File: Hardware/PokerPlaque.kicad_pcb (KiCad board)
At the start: 2 copper layers, 43.1 x 40.2 mm, 10 parts, among them J1 A2541WR-5P, J2 A2541WR-4P, J3 A2541WR-2P, J4 A2541WR-8P, SW1 KH-6X6X6H-STM, U1 CH32V203C8T6

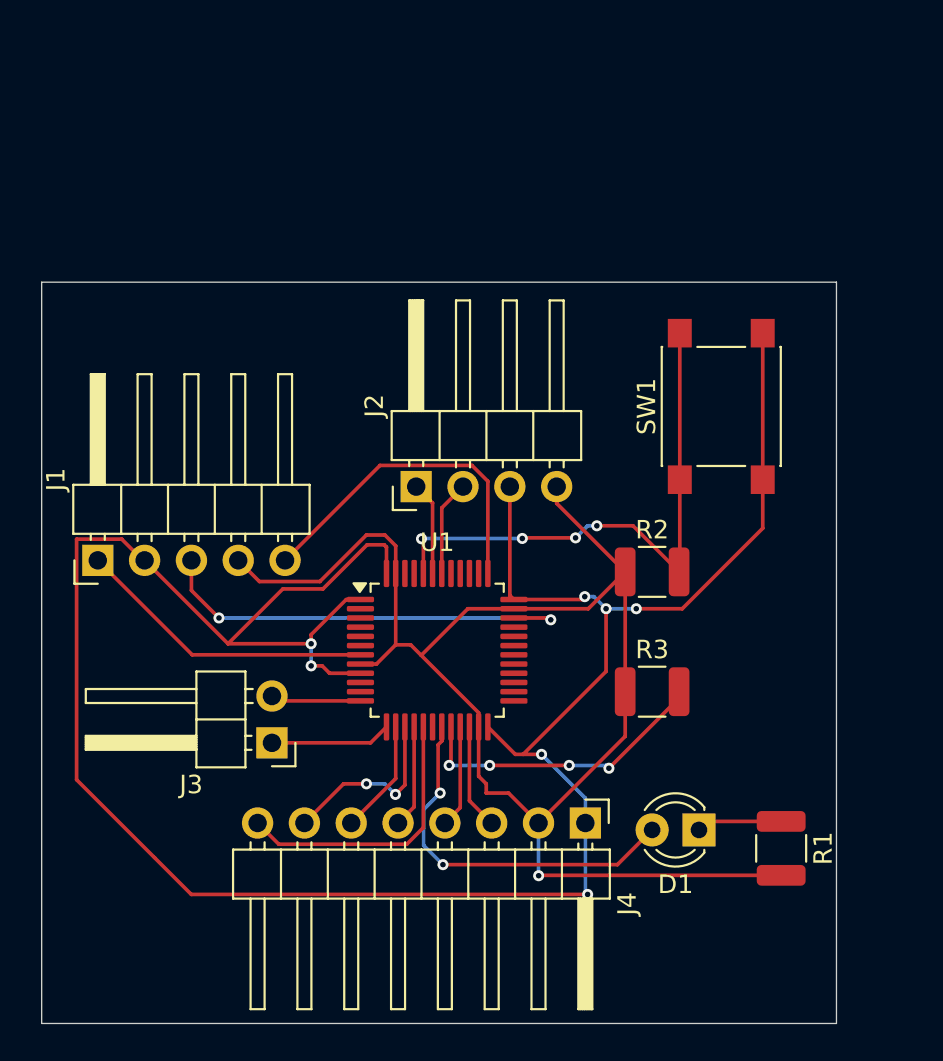
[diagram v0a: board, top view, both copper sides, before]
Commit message: feat: more things
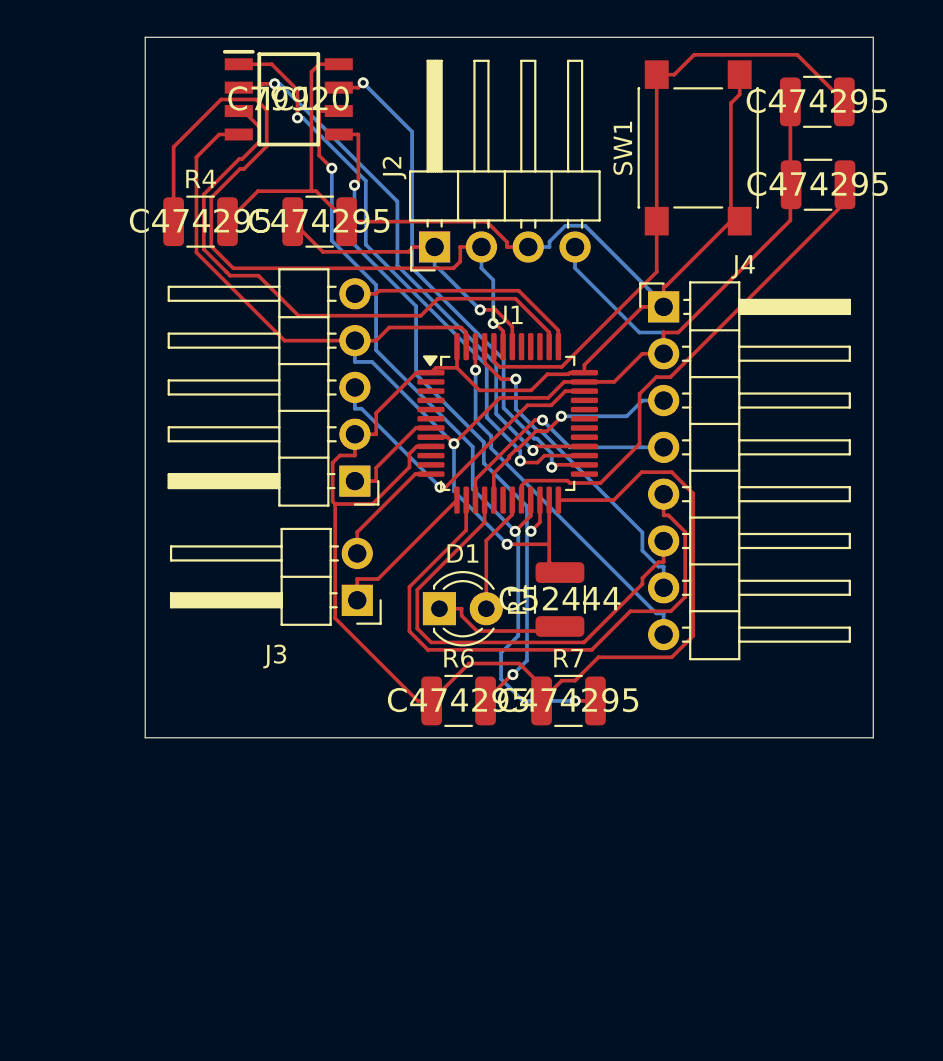
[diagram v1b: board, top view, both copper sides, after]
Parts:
- added IC1: M24C32-RMN6TP, M24C32-RMN6TP:SOIC127P600X175-8N, F.Cu at (35.3, 18.9)
- added R4: 1210W2J0103T5E, Resistor_SMD:R_1210_3225Metric, F.Cu at (30.5, 25.5)
- added R5: 1210W2J0103T5E, Resistor_SMD:R_1210_3225Metric, F.Cu at (37.0, 25.5)
- added R6: 1210W2J0103T5E, Resistor_SMD:R_1210_3225Metric, F.Cu at (44.5, 51.5)
- added R7: 1210W2J0103T5E, Resistor_SMD:R_1210_3225Metric, F.Cu at (50.5, 51.5)
- R1: value 1k Ohm -> 1210W2F1001T5E
- R2, R3: value 10k Ohm -> 1210W2J0103T5E
- moved R3 28.9 mm to (64.0, 23.5)
- moved J4 28.3 mm to (55.6, 30.1), turned to 0 degrees
- moved R2 27.0 mm to (64.0, 19.0)
- moved D1 18.5 mm to (43.5, 46.5), turned to 0 degrees
- moved R1 18.1 mm to (50.0, 46.0), turned to 90 degrees
- moved J1 14.6 mm to (38.9, 39.6), turned to 180 degrees
- moved SW1 14.1 mm to (57.5, 21.5)
- moved J2 13.0 mm to (43.2, 26.9)
- moved U1 12.9 mm to (47.2, 36.4)
- moved J3 9.01 mm to (39.0, 46.0)
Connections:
- J2 pad 1: I2C1_SDA -> I2C1_SCL
- J2 pad 2: I2C1_SCL -> I2C1_SDA
- J4 pad 3: DISPLAY_BUSY -> DISPLAY_MOSI1
- J4 pad 4: DISPLAY_RESET -> DISPLAY_SCK1
- J4 pad 5: DISPLAY_MISO1 -> DISPLAY_SS1
- J4 pad 6: DISPLAY_SS1 -> DISPLAY_MISO1
- J4 pad 7: DISPLAY_SCK1 -> DISPLAY_RESET
- J4 pad 8: DISPLAY_MOSI1 -> DISPLAY_BUSY
- U1 pad 21: DISPLAY_RESET -> EEPROM_I2C2_SCL
- U1 pad 22: DISPLAY_BUSY -> EEPROM_I2C2_SDA
- U1 pad 26: unconnected-(U1-PB13-Pad26) -> EEPROM_I2C2_WC
- U1 pad 27: unconnected-(U1-PB14-Pad27) -> EEPROM_E0
- U1 pad 28: unconnected-(U1-PB15-Pad28) -> EEPROM_E1
- U1 pad 38: unconnected-(U1-PA15-Pad38) -> EEPROM_E2
- U1 pad 45: unconnected-(U1-PB8-Pad45) -> DISPLAY_RESET
- U1 pad 46: unconnected-(U1-PB9-Pad46) -> DISPLAY_BUSY
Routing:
- net EEPROM_I2C2_SCL: track 0.00 -> 44.4 mm, vias 0 -> 3
- net EEPROM_I2C2_SDA: track 0.00 -> 38.8 mm, vias 0 -> 3
- net I2C1_SDA: track 5.08 -> 41.2 mm, vias 0 -> 1
- net EEPROM_E0: track 0.00 -> 32.7 mm, vias 0 -> 2
- net EEPROM_E2: track 0.00 -> 31.6 mm
- net EEPROM_E1: track 0.00 -> 30.8 mm, vias 0 -> 2
- net EEPROM_I2C2_WC: track 0.00 -> 28.4 mm, vias 0 -> 2
- net DISPLAY_SS1: track 6.21 -> 31.2 mm
- net DISPLAY_MISO1: track 5.57 -> 25.3 mm
- net DISPLAY_BUSY: track 5.71 -> 20.1 mm, vias 0 -> 1
- net DEBUG_LED0: track 20.5 -> 6.48 mm, vias 2 -> 0
- net DISPLAY_RESET: track 5.56 -> 17.9 mm, vias 0 -> 1
- net I2C1_SCL: track 5.19 -> 16.3 mm, vias 0 -> 1
- net BOOT1: track 16.6 -> 27.4 mm, vias 4 -> 0
- net RST: track 16.4 -> 5.74 mm
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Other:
- board size 43.1 x 40.2 mm -> 39.5 x 38 mm
